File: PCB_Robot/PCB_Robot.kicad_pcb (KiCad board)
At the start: 2 copper layers, 15 parts, among them J1 UART, J2 Alimentacion, J3 MotorL, J4 MotorR, U1 ESP32-WROOM-E, U2 TB6612FNG, U3 BMI160

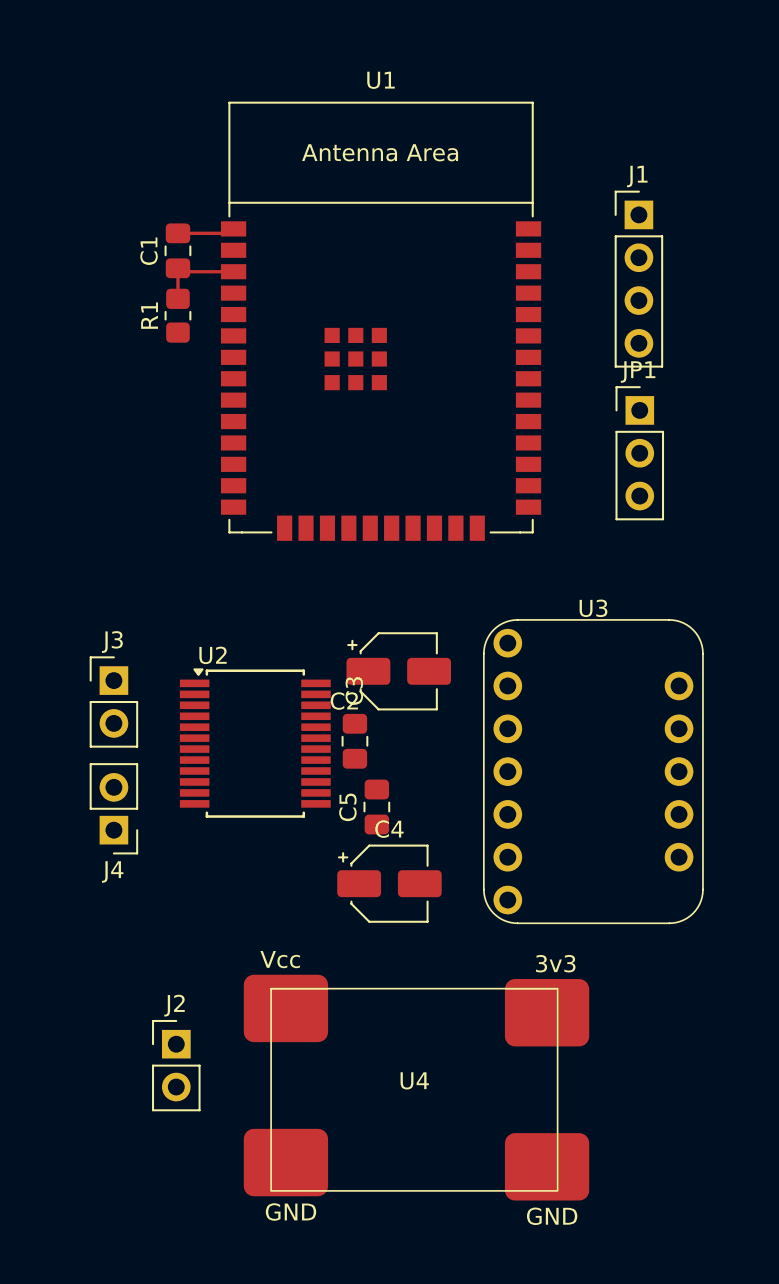
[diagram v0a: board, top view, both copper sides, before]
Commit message: PCB Actualizda
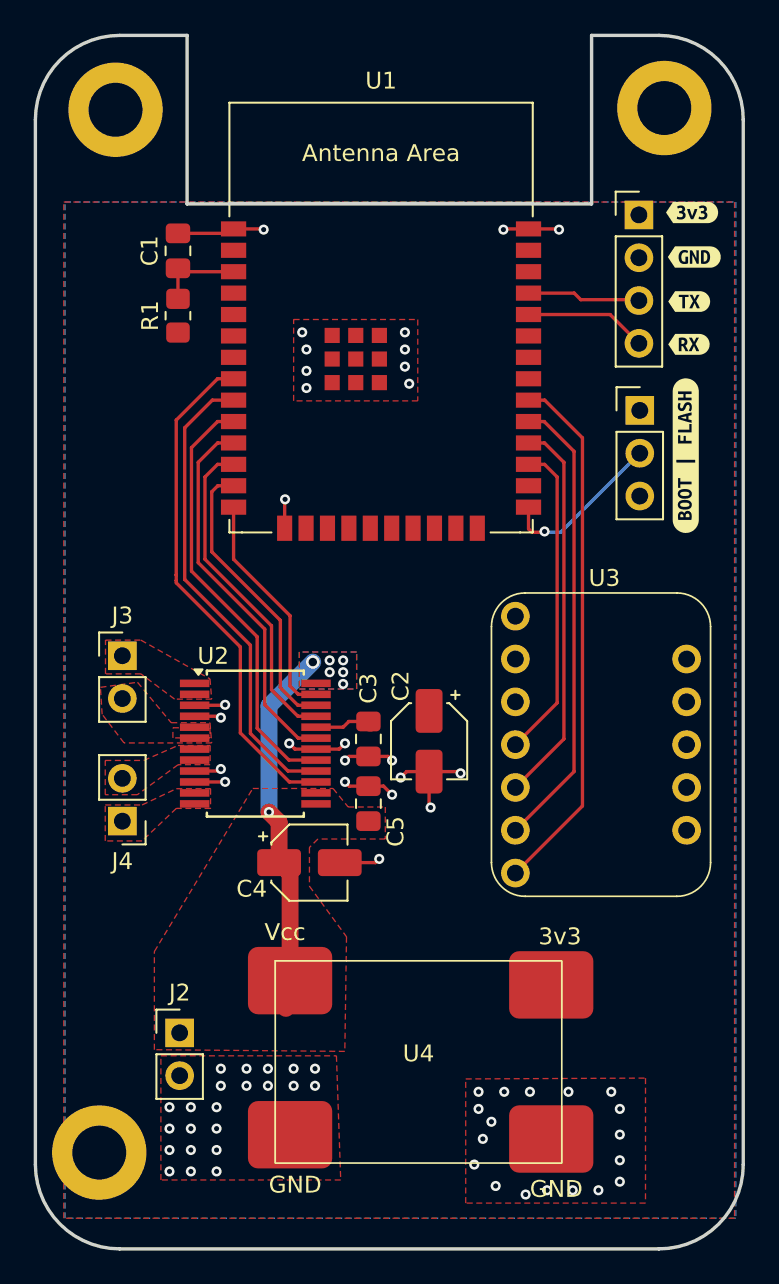
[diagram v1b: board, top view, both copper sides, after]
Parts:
- added REF**: MountingHole_3.2mm_M3_DIN965_Pad, MountingHole:MountingHole_3.2mm_M3_DIN965_Pad, F.Cu at (149.8, 74.8)
- added REF**: MountingHole_3.2mm_M3_DIN965_Pad, MountingHole:MountingHole_3.2mm_M3_DIN965_Pad, F.Cu at (116.2, 136.8)
- added REF**: MountingHole_3.2mm_M3_DIN965_Pad, MountingHole:MountingHole_3.2mm_M3_DIN965_Pad, F.Cu at (117.2, 74.9)
- added REF**: KiCad-Logo2_6mm_SilkScreen, Symbol:KiCad-Logo2_6mm_SilkScreen, B.Cu at (135.8, 127.0)
- added kibuzzard-684B1A20: G***, kibuzzard-684B1A20, F.Cu at (151.5, 83.7)
- added kibuzzard-684B1A93: G***, kibuzzard-684B1A93, F.Cu at (151.0, 95.5)
- added kibuzzard-684B1AB0: G***, kibuzzard-684B1AB0, F.Cu at (151.2, 86.3)
- added kibuzzard-684B1AB8: G***, kibuzzard-684B1AB8, F.Cu at (151.2, 88.8)
- added kibuzzard-684B1AD4: G***, kibuzzard-684B1AD4, F.Cu at (151.4, 81.0)
- moved C4 4.91 mm to (128.7, 119.6)
- moved C2 4.52 mm to (135.8, 112.4), turned to -90 degrees
- moved U4 1.67 mm to (135.2, 131.4)
- moved U3 1.66 mm to (146.0, 112.6)
- moved J3 1.56 mm to (117.6, 107.3)
- moved C3 0.81 mm to (132.2, 112.3)
- moved J4 0.73 mm to (117.6, 117.1)
- moved J2 0.70 mm to (121.0, 129.7)
- moved C5 0.54 mm to (132.2, 116.1)
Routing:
- net GND: track 3.41 -> 35.1 mm, vias 0 -> 66
- net /BMI_MISO: track 0.00 -> 31.6 mm
- net /MT_PWMB: track 0.00 -> 30.3 mm
- net /MT_BIN2: track 0.00 -> 28.1 mm
- net /BMI_CS: track 0.00 -> 27.4 mm
- net /MT_BIN1: track 0.00 -> 25.7 mm
- net /BMI_MOSI: track 0.00 -> 23.1 mm
- net /MT_STBY: track 0.00 -> 22.5 mm
- net /V_MOTOR: track 0.00 -> 20.6 mm, vias 0 -> 7
- net /MT_AIN1: track 0.00 -> 19.6 mm
- net /BMI_SCK: track 0.00 -> 18.9 mm
- net /MT_AIN2: track 0.00 -> 17.3 mm
- net /MT_PWMA: track 0.00 -> 13.7 mm
- net Net-(JP1-C): track 0.00 -> 9.96 mm, vias 0 -> 1
- net Net-(J1-Pin_4): track 0.00 -> 7.26 mm
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- added copper zone on F.Cu, net +3V3
- added copper zone on B.Cu, net /V_MOTOR
- added copper zone on F.Cu, net /V_MOTOR
- added copper zone on B.Cu, net GND
- added copper zone on F.Cu, net GND
- added copper zone on F.Cu, net Net-(J3-Pin_1)
- added copper zone on F.Cu, net Net-(J3-Pin_2)
- added copper zone on F.Cu, net Net-(J4-Pin_1)
- added copper zone on F.Cu, net Net-(J4-Pin_2)
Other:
- board outline added: 42 x 72 mm
